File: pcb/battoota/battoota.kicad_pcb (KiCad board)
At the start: 2 copper layers, 124.7 x 97.3 mm, 38 parts

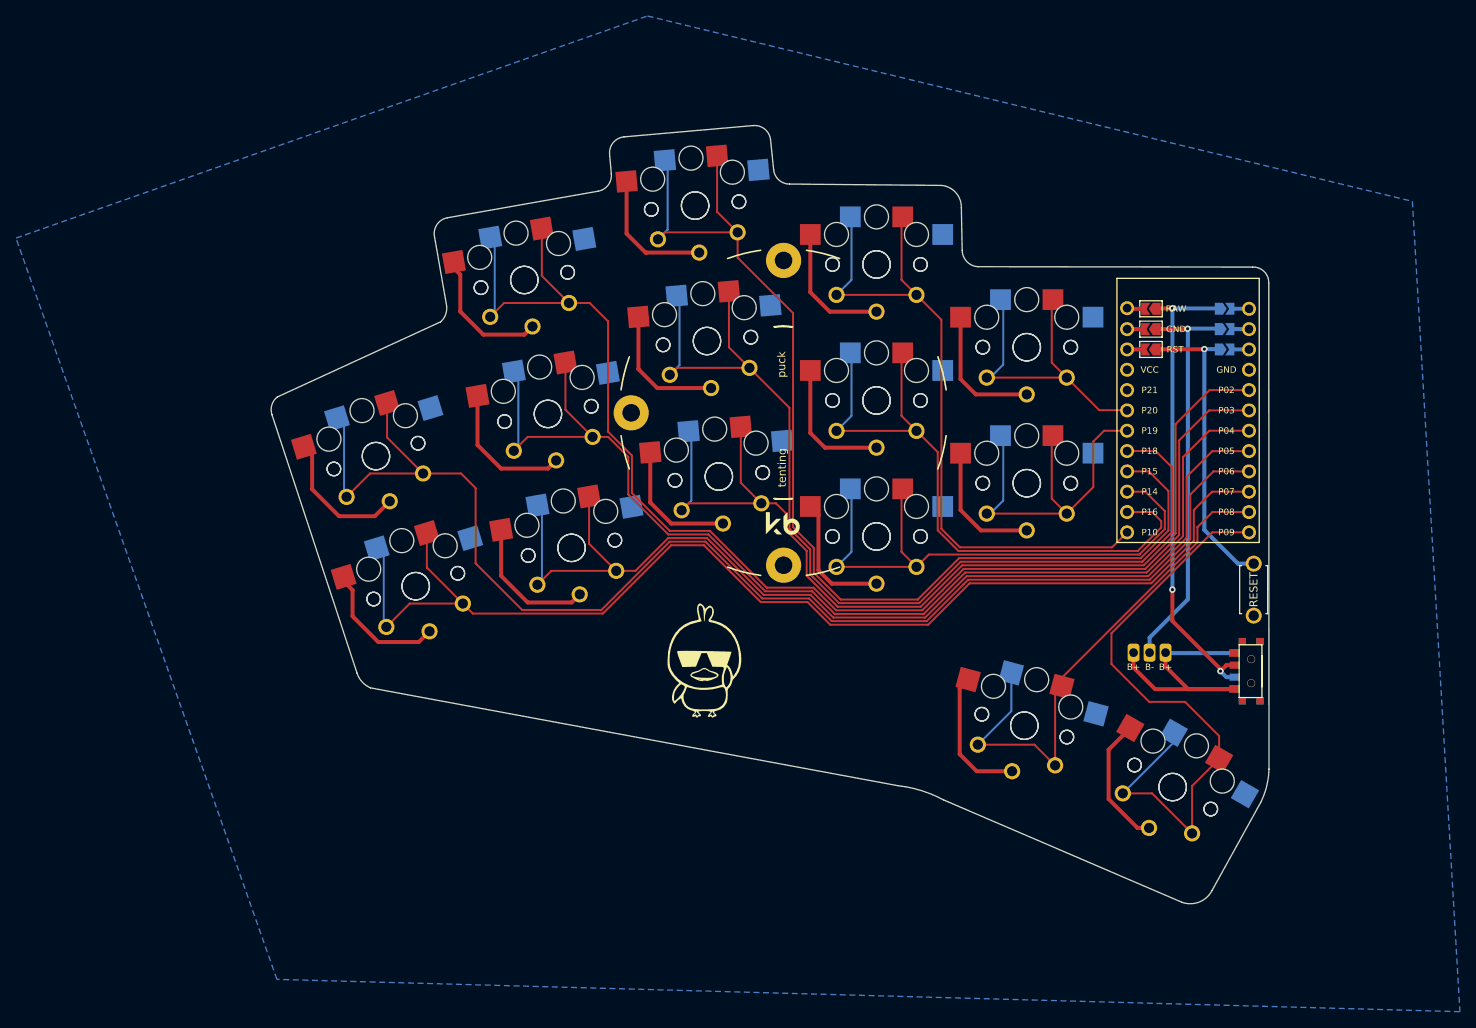
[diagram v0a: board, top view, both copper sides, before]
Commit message: pcb shape change
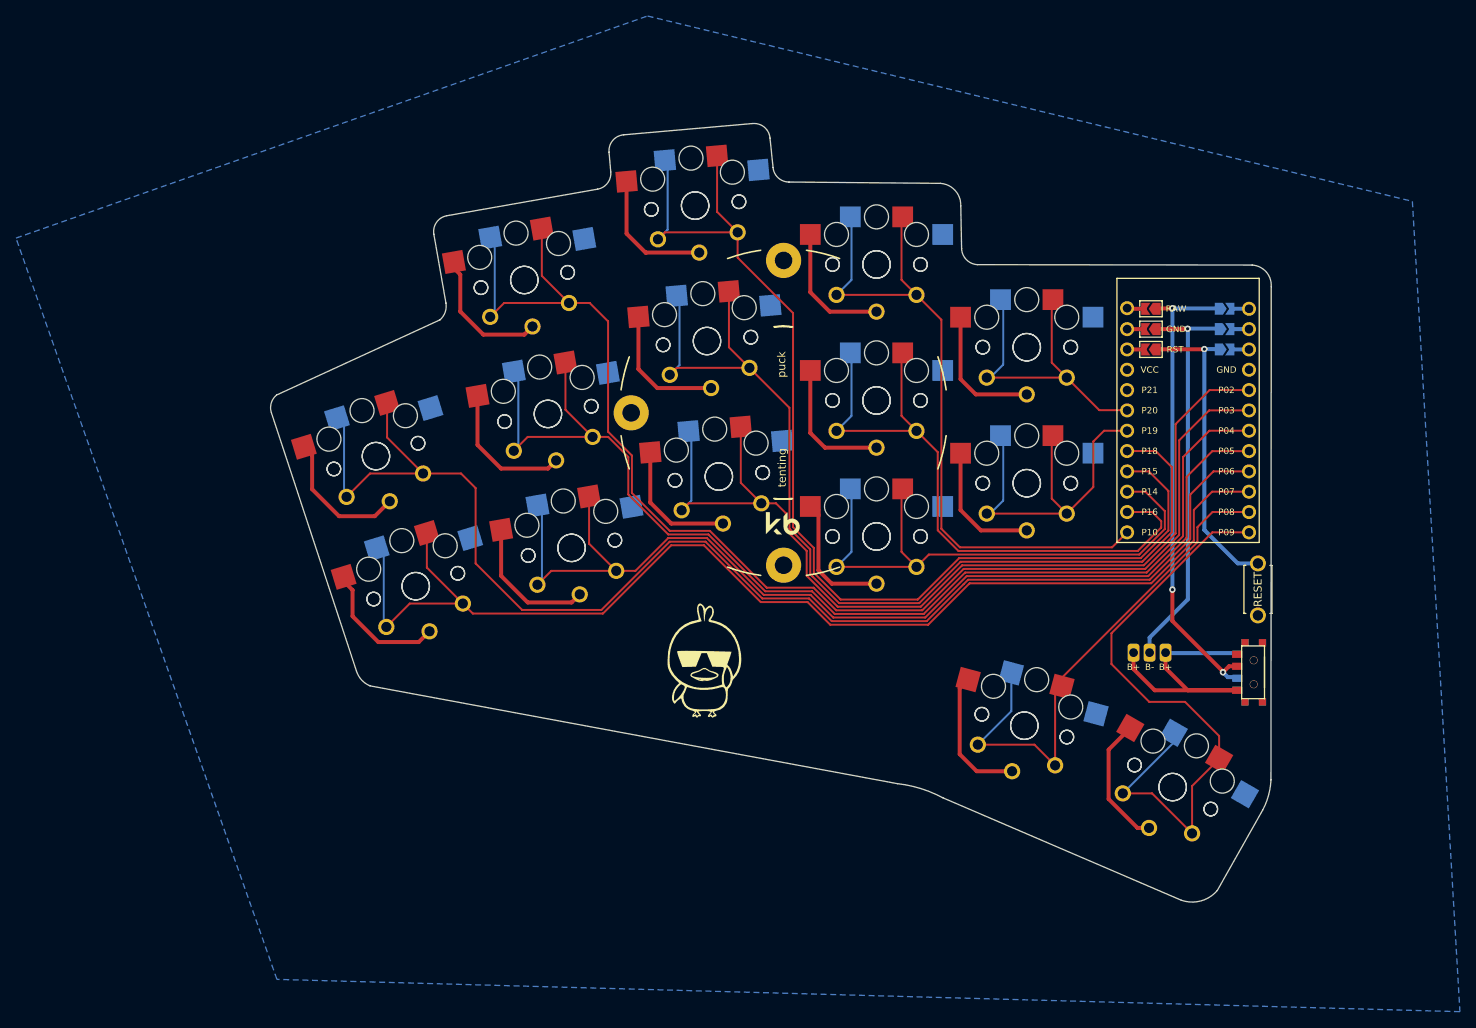
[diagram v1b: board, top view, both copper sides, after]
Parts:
- moved B1 0.53 mm to (163.1, -66.1)
- moved T1 0.35 mm to (162.6, -55.7)
- moved T2 0.35 mm to (162.6, -55.7)
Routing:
- net Braw: track 35.8 -> 37.1 mm
- net RST: track 38.3 -> 38.8 mm
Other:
- board size 124.7 x 97.3 mm -> 125.1 x 97.3 mm
